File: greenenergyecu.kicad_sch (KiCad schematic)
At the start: 35 parts, among them J22 USB_B_Mini, M1 Module-power_12and5V-0.3, M2 Module-knock-0.2, M3 Module-vr-discrete-0.5, M4 Module-vr-max9924-0.1, M5 Module-wbo-0.5, M6 Module:mega-mcu100/0.3, M7 Module-can-0.1, M8 Module-motor-driver-0.1, P1 368255-2, Q1 AO3400A, U1 BTS6143D

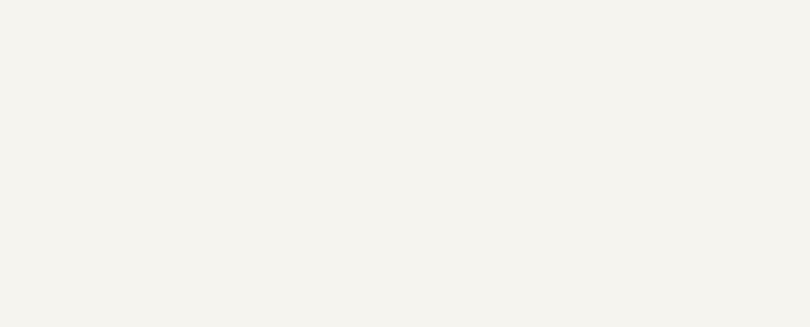
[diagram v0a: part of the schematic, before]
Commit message: weew
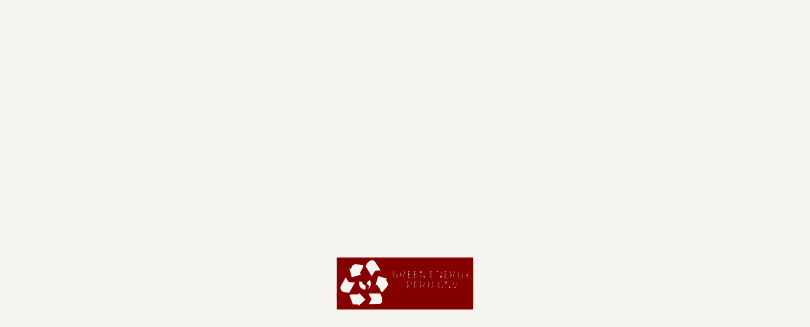
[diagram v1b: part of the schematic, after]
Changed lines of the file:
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@@
+	)
+	(symbol
+		(lib_name "LOGO_1")
+		(lib_id "lokon:LOGO")
+		(at 367.03 407.67 0)
+		(unit 1)
+		(exclude_from_sim no)
+		(in_bom yes)
+		(on_board yes)
+		(dnp no)
+		(fields_autoplaced yes)
+		(property "Reference" "#G2"
+			(at 367.03 405.5029 0)
+			(effects
+				(font
+					(size 1.27 1.27)
+				)
+				(hide yes)
+			)
+		)
+		(property "Value" "LOGO"
+			(at 367.03 409.8371 0)
+			(effects
+				(font
+					(size 1.27 1.27)
+				)
+				(hide yes)
+			)
+		)
+		(property "Footprint" ""
+			(at 367.03 407.67 0)
+			(effects
+				(font
+					(size 1.27 1.27)
+				)
+				(hide yes)
+			)
+		)
+		(property "Datasheet" ""
+			(at 367.03 407.67 0)
+			(effects
+				(font
+					(size 1.27 1.27)
+				)
+				(hide yes)
+			)
+		)
+		(property "Description" ""
+			(at 367.03 407.67 0)
+			(effects
+				(font
+					(size 1.27 1.27)
+				)
+				(hide yes)
+			)
+		)
+		(instances
+			(project ""
+				(path "/45c1f041-3b7c-4036-abe9-e26621c05a73"
+					(reference "#G2")
+					(unit 1)
+				)
+			)
+		)
 	)
 	(symbol
